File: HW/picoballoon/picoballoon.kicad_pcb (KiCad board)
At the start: 4 copper layers, 58.4 x 42 mm, 87 parts, among them J1 EXT_DEBUGGER, U1 Si4461, U2 MPL3115A2, U4 MCP9802, U5 MAX-M10S, U6 OPA333xxDBV, Y1 30M

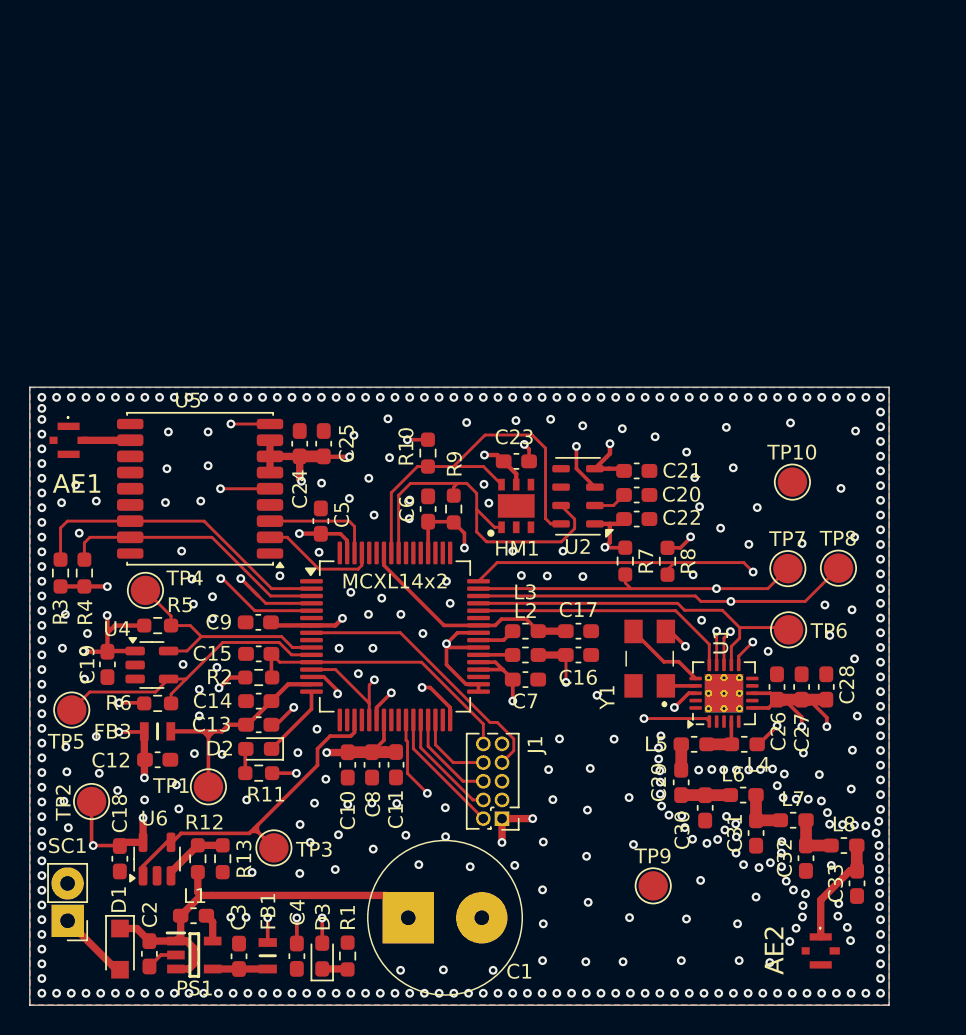
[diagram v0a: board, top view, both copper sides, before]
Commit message: mcxc
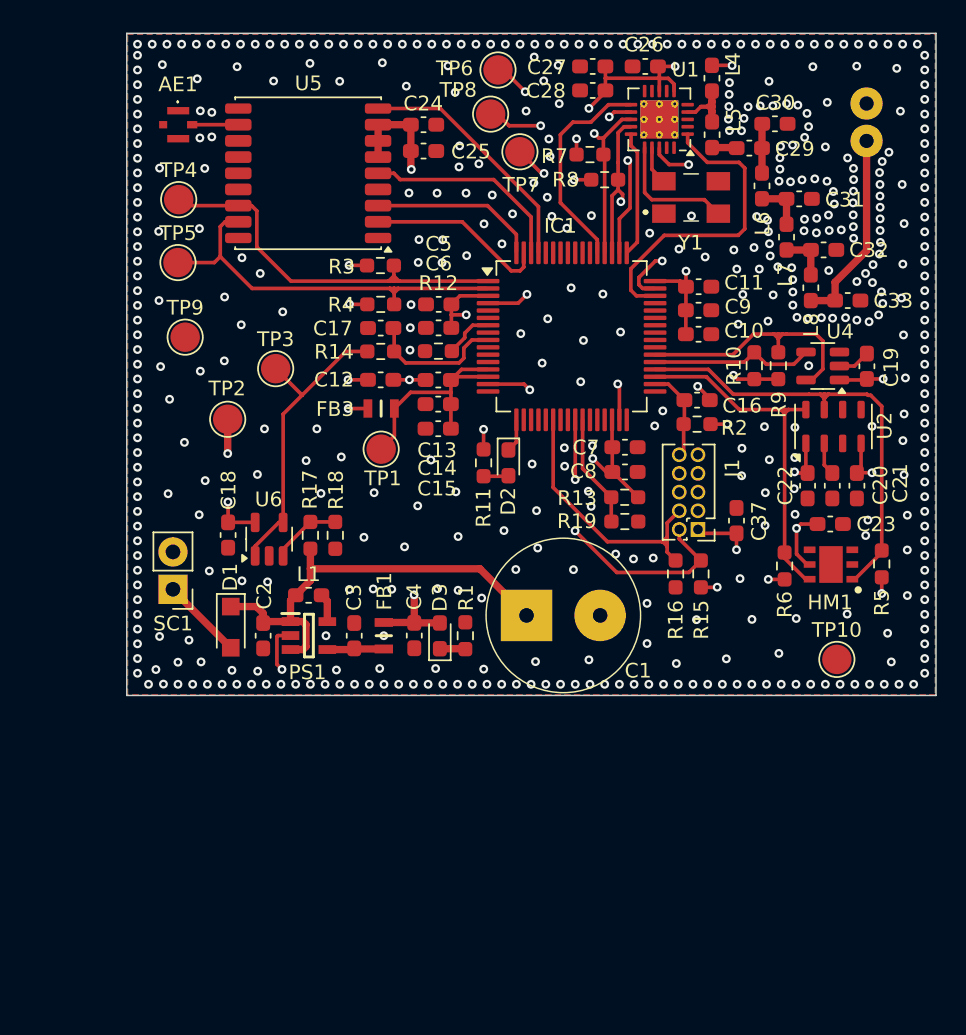
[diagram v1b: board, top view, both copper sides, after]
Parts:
- removed the ? at (148.4, 128.9)
- removed the ? at (147.4, 128.9)
- removed the ? at (147.4, 129.9)
- removed the ? at (146.3, 128.9)
- removed the ? at (147.4, 127.8)
- removed L2, L3: 4.7u, Inductor_SMD:L_0603_1608Metric_Pad1.05x0.95mm_HandSolder
- removed MCXL14x2: ~, Package_QFP:LQFP-64-1EP_10x10mm_P0.5mm_EP5x5mm
- added ?: , , F.Cu at (141.9, 89.8)
- added ?: , , F.Cu at (143.0, 89.9)
- added ?: , , F.Cu at (143.0, 88.8)
- added ?: , , F.Cu at (144.0, 89.8)
- added ?: , , F.Cu at (143.0, 90.9)
- added C37: 100n, Capacitor_SMD:C_0603_1608Metric_Pad1.08x0.95mm_HandSolder, F.Cu at (148.2, 117.1)
- added IC1: MCXC141VLH, Package_QFP:LQFP-64-1EP_10x10mm_P0.5mm_EP5x5mm, F.Cu at (137.0, 104.6)
- added R14: 1k, Resistor_SMD:R_0603_1608Metric_Pad0.98x0.95mm_HandSolder, F.Cu at (124.0, 105.6)
- added R15: 10k, Resistor_SMD:R_0603_1608Metric_Pad0.98x0.95mm_HandSolder, F.Cu at (145.8, 120.8)
- added R16: 10k, Resistor_SMD:R_0603_1608Metric_Pad0.98x0.95mm_HandSolder, F.Cu at (144.1, 120.8)
- added R17: 1M, Resistor_SMD:R_0603_1608Metric_Pad0.98x0.95mm_HandSolder, F.Cu at (119.2, 118.1)
- added R18: 1M, Resistor_SMD:R_0603_1608Metric_Pad0.98x0.95mm_HandSolder, F.Cu at (120.9, 118.1)
- added R19: 0, Resistor_SMD:R_0603_1608Metric_Pad0.98x0.95mm_HandSolder, F.Cu at (140.6, 117.2)
- AE2: footprint Library:RECE20369001E01 -> Library:BNC_Connector_PCB
- C10, C6, C8: value 100n -> 1u
- C16: value 4.7u -> 100n
- C17: value 4.7u -> xx
- R12, R13: value 1M -> 10k
- moved C19 55.4 mm to (157.1, 106.6), turned to 90 degrees
- moved AE2 55.1 mm to (157.1, 91.3), turned to 90 degrees
- moved U4 49.9 mm to (154.1, 106.6), turned to 180 degrees
- moved R5 49.4 mm to (158.1, 120.1), turned to -90 degrees
- moved TP9 49.0 mm to (110.7, 104.7)
- moved C30 46.7 mm to (150.8, 90.2), turned to 180 degrees
- moved L4 45.3 mm to (146.5, 87.1), turned to -90 degrees
- moved C27 44.5 mm to (138.4, 86.3), turned to 180 degrees
- moved R6 43.6 mm to (151.5, 120.2), turned to -90 degrees
- moved C28 43.5 mm to (138.4, 87.9), turned to 180 degrees
- moved C29 43.4 mm to (149.1, 91.8), turned to 0 degrees
- moved C31 43.2 mm to (152.5, 95.3), turned to 180 degrees
- moved C26 43.1 mm to (142.0, 86.3), turned to 180 degrees
- moved TP6 42.9 mm to (132.0, 86.5)
- moved L5 41.4 mm to (146.6, 90.9), turned to -90 degrees
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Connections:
- AE1 pad 2: GND -> (no net)
- AE1 pad 3: GND -> (no net)
- AE1 pad 4: GND -> (no net)
- AE2 pad 2: GND -> (no net)
- C15 pad 1: /RESET -> +3.3VA
- C16 pad 1: /VDD_CORE -> /RESET
- C17 pad 1: /VDD_CORE_1POV -> Net-(IC1-PTE20)
- J1 pad 2: Net-(J1-Pin_2) -> /SWD_DIO
- J1 pad 4: Net-(J1-Pin_4) -> /SWD_CLK
- J1 pad 6: Net-(J1-Pin_6) -> unconnected-(J1-Pin_6-Pad6)
- J1 pad 7: /ISP -> unconnected-(J1-Pin_7-Pad7)
- J1 pad 8: Net-(J1-Pin_8) -> unconnected-(J1-Pin_8-Pad8)
- R10 pad 1: +3.3V -> /SCL_TEMP
- R10 pad 2: /SCL_SENS -> +3.3V
- R12 pad 1: +U_SC -> Net-(IC1-PTE18)
- R12 pad 2: Net-(U6-+) -> GND
- R13 pad 1: Net-(U6-+) -> +3.3V
- R13 pad 2: GND -> Net-(IC1-PTA4)
- R5 pad 1: +3.3V -> /SDA_SENS
- R5 pad 2: /SDA_TEMP -> +3.3V
- R6 pad 1: +3.3V -> /SCL_SENS
- R6 pad 2: /SCL_TEMP -> +3.3V
- R7 pad 2: /MOSI -> /MISO
- R8 pad 2: /nIRQ -> /MOSI
- R9 pad 1: +3.3V -> /SDA_TEMP
- R9 pad 2: /SDA_SENS -> +3.3V
- TP4 pad 1: /SDA_TEMP -> /GNSS_SDA
- TP5 pad 1: /SCL_TEMP -> /GNSS_SCL
- Y1 pad 3: GND -> (no net)
- Y1 pad 4: GND -> (no net)
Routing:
- net /VDD_CORE: track 24.8 -> 0.00 mm, vias 2 -> 0
- net +3.3V: track 107.0 -> 84.9 mm, vias 30 -> 27
- net /SWD_DIO: track 0.00 -> 20.5 mm, vias 0 -> 2
- net /SWD_CLK: track 0.00 -> 18.7 mm
- net /ISP: track 18.7 -> 0.00 mm
- net /VDD_CORE_1POV: track 15.4 -> 0.00 mm
- net /RESET: track 19.4 -> 6.30 mm
- net /nIRQ: track 27.2 -> 14.7 mm, vias 2 -> 0
- net /MISO: track 30.1 -> 18.4 mm
- net /nSEL: track 18.0 -> 8.54 mm
- net /SCL_TEMP: track 20.6 -> 11.2 mm
- net Net-(IC1-PTE20): track 0.00 -> 9.30 mm
- net /MOSI: track 27.9 -> 18.6 mm
- net /GNSS_SCL: track 18.4 -> 27.4 mm
- net Net-(J1-Pin_2): track 8.68 -> 0.00 mm
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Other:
- board size 58.4 x 42 mm -> 55 x 45 mm
